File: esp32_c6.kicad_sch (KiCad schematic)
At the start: 43 parts, among them J21 USB_B_Mini, J6 FT232RL, Q4 Q_NPN_BCE, Q5 Q_PNP_BCE, SW1 SW_Push, SW11 boot, U1 ESP32-C6-WROOM-1-N8, U2 ESP32-C6-DEVKITC-1-N8, U9 LM1117DT-3.3, Y2 Two pin oscilador 32768hz

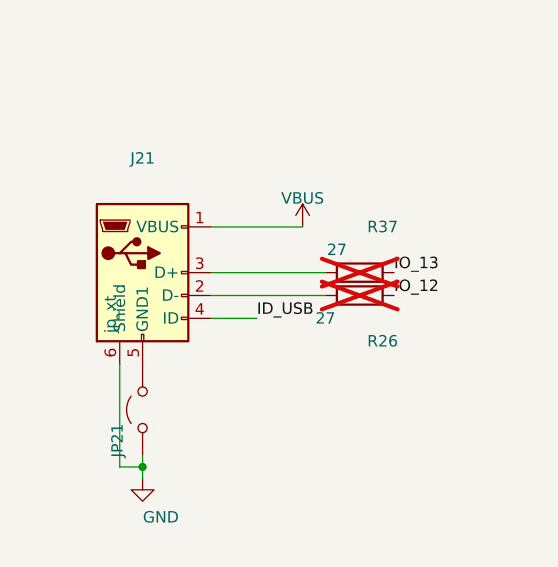
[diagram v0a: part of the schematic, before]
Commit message: add update
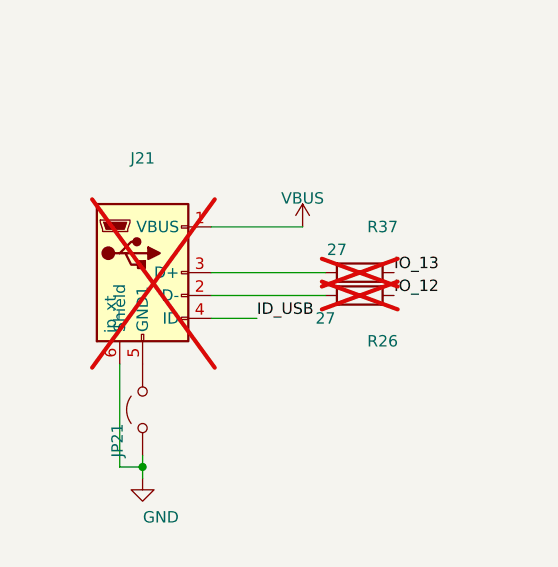
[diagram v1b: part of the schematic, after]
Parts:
- J21: now not fitted
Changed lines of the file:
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@@
 		(on_board yes)
 		(in_pos_files no)
-		(dnp no)
+		(dnp yes)
 		(fields_autoplaced yes)
 		(property "Reference" "J21"

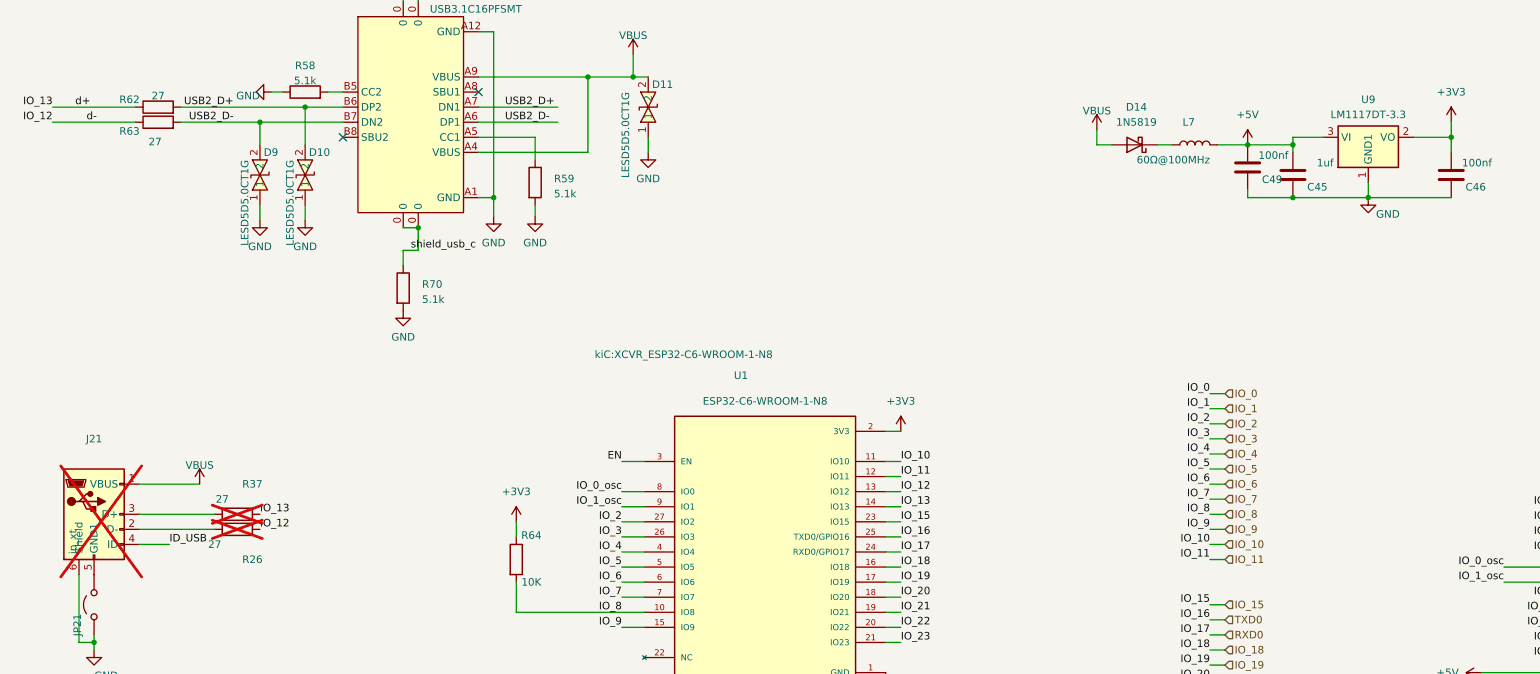
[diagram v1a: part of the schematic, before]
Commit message: correccion de partes
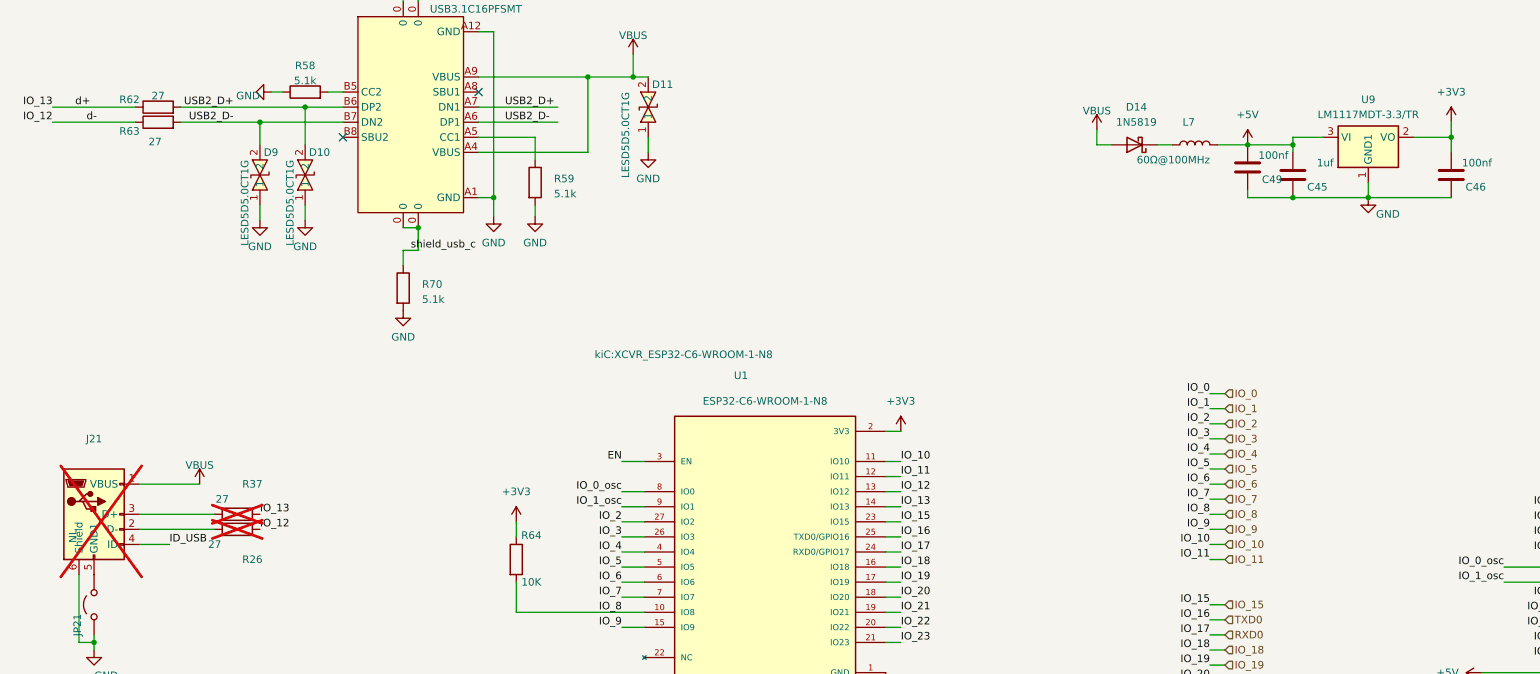
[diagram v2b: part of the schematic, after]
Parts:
- J21: value USB_B_Mini -> U-M-M5SS-W-2
- JP21: value jp_xt -> NL
- U9: value LM1117DT-3.3 -> LM1117MDT-3.3/TR; LCSC C969102 -> C498159
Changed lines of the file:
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@@
 			)
 		)
-		(property "Value" "USB_B_Mini"
+		(property "Value" "U-M-M5SS-W-2"
 			(at 55.88 106.68 0)
 			(hide yes)
@@
 			)
 		)
-		(property "Value" "LM1117DT-3.3"
+		(property "Value" "LM1117MDT-3.3/TR"
 			(at 270.51 49.53 0)
 			(show_name no)
@@
 			)
 		)
-		(property "LCSC" "C969102"
+		(property "LCSC" "C498159"
 			(at 270.51 53.34 0)
 			(hide yes)
@@
 		(in_bom no)
 		(on_board yes)
-		(in_pos_files yes)
+		(in_pos_files no)
 		(dnp no)
 		(property "Reference" "JP21"
@@
 			)
 		)
-		(property "Value" "jp_xt"
+		(property "Value" "NL"
 			(at 52.324 119.38 0)
 			(show_name no)
